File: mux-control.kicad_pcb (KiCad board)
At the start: 2 copper layers, 14 parts, among them J1 Conn_01x08, SW1 SW_Push_Dual, SW2 SW_Push_Dual, SW3 SW_Push_Dual, SW4 SW_Push_Dual, U1 CD74HC4051E

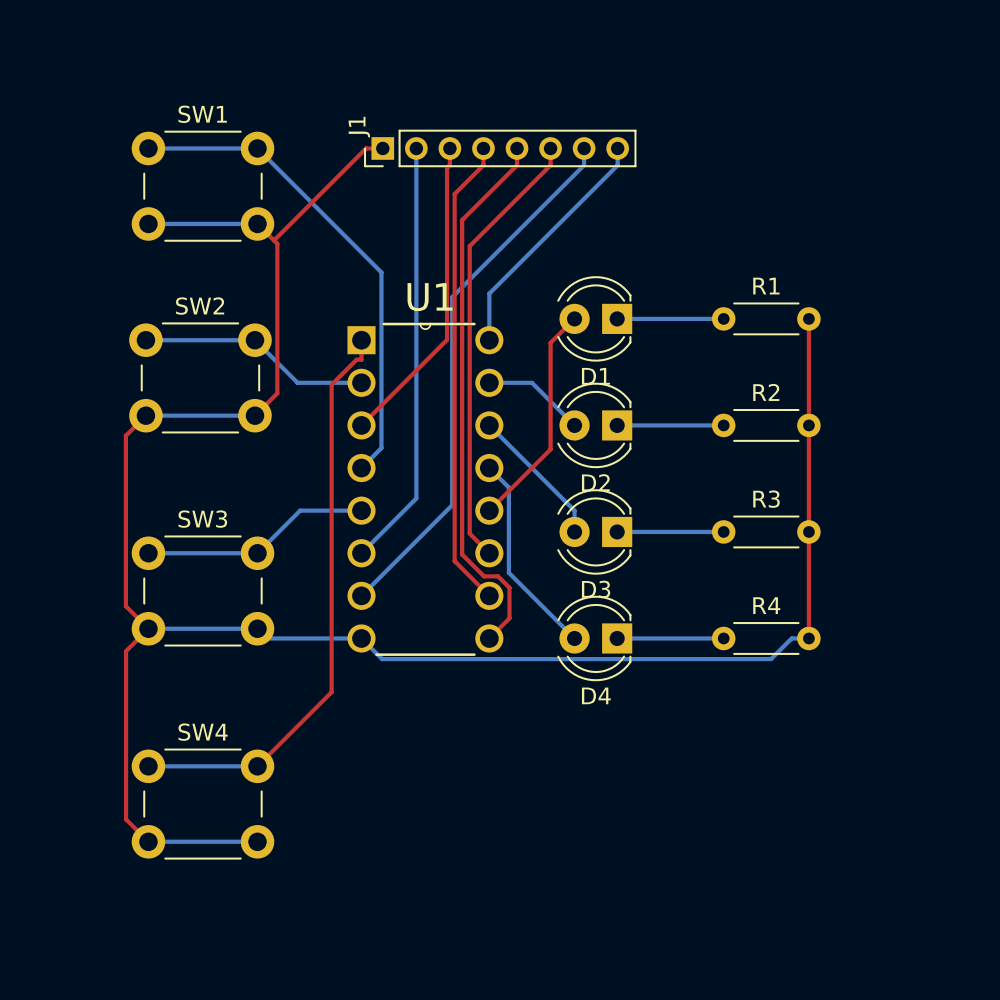
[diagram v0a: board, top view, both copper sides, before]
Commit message: new design
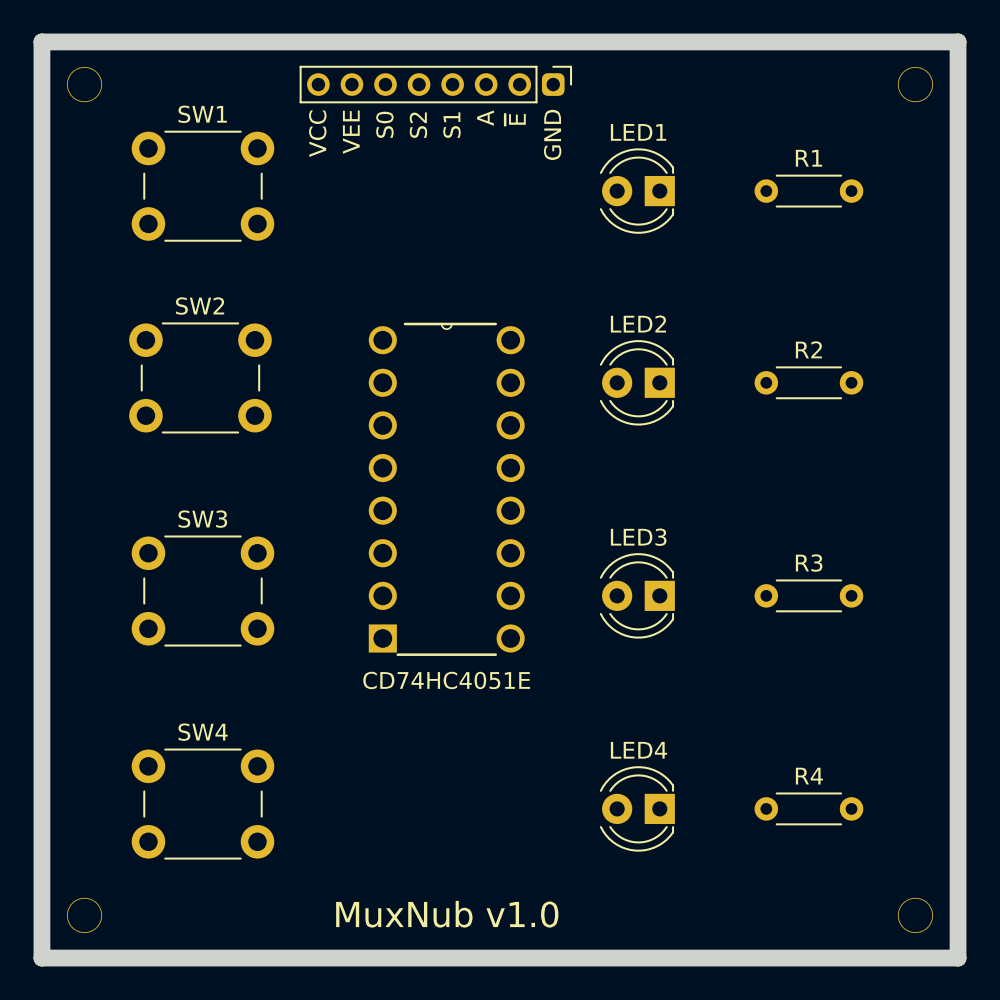
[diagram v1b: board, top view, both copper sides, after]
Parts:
- added MO1: M1, MountingHole:MountingHole_2.1mm, F.Cu at (121.9, 62.2)
- added MO2: , MountingHole:MountingHole_2.1mm, F.Cu at (121.9, 111.8)
- added MO3: , MountingHole:MountingHole_2.1mm, F.Cu at (171.4, 62.2)
- added MO4: , MountingHole:MountingHole_2.1mm, F.Cu at (171.4, 111.8)
- D1: value LED -> LED1
- D2: value LED -> LED2
- D3: value LED -> LED3
- D4: value LED -> LED4
- moved J1 10.9 mm to (149.9, 62.2), turned to 270 degrees
- moved D4 10.5 mm to (156.2, 105.4)
- moved R4 10.5 mm to (162.6, 105.4)
- moved D1 8.03 mm to (156.2, 68.6)
- moved R1 8.03 mm to (162.6, 68.6)
- moved D3 4.58 mm to (156.2, 92.7)
- moved R3 4.58 mm to (162.6, 92.7)
- moved D2 3.59 mm to (156.2, 80.0)
- moved R2 3.59 mm to (162.6, 80.0)
- moved U1 1.27 mm to (147.3, 95.2)
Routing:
- net Net-(J1-Pad1): track 128.0 -> 0.00 mm
- net Net-(SW4-Pad1): track 34.6 -> 0.00 mm
- net Net-(J1-Pad5): track 32.7 -> 0.00 mm
- net Net-(J1-Pad7): track 32.2 -> 0.00 mm
- net Net-(SW1-Pad1): track 29.1 -> 0.00 mm
- net Net-(J1-Pad4): track 28.2 -> 0.00 mm
- net Net-(J1-Pad6): track 26.6 -> 0.00 mm
- net Net-(J1-Pad2): track 25.5 -> 0.00 mm
- net Net-(J1-Pad3): track 18.7 -> 0.00 mm
- net Net-(J1-Pad8): track 14.6 -> 0.00 mm
- net Net-(SW2-Pad1): track 13.9 -> 0.00 mm
- net Net-(SW3-Pad1): track 13.8 -> 0.00 mm
- net Net-(D1-Pad2): track 13.5 -> 0.00 mm
- net Net-(D4-Pad2): track 12.3 -> 0.00 mm
- net Net-(D3-Pad2): track 8.45 -> 0.00 mm
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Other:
- board outline added: 54.6 x 54.6 mm
- board text added: "MuxNub v1.0"
